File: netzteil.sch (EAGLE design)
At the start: 49 parts, among them X1 NEB21R

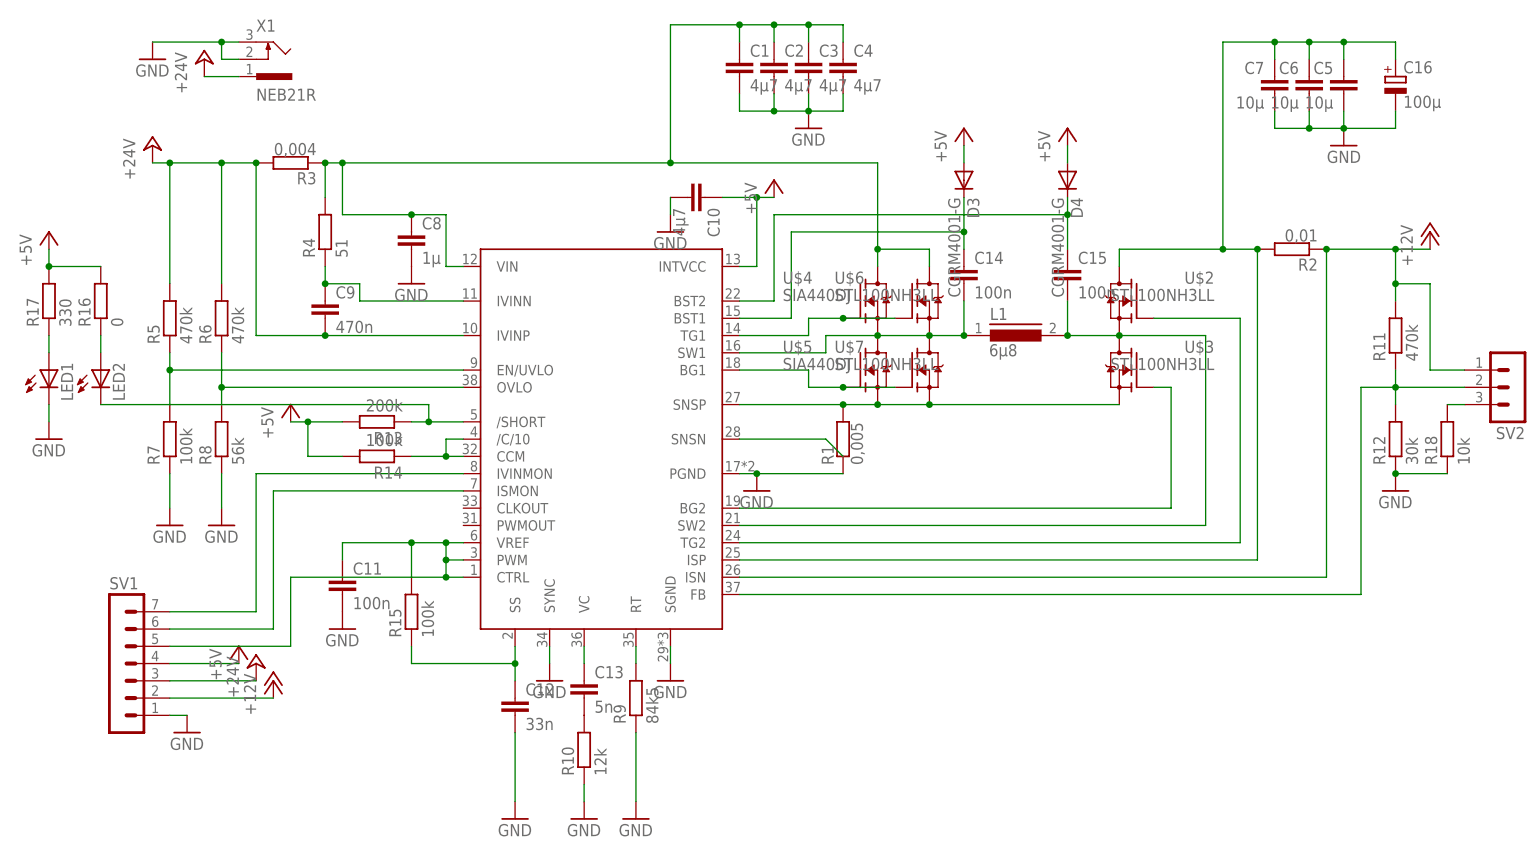
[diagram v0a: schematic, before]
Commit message: version 2
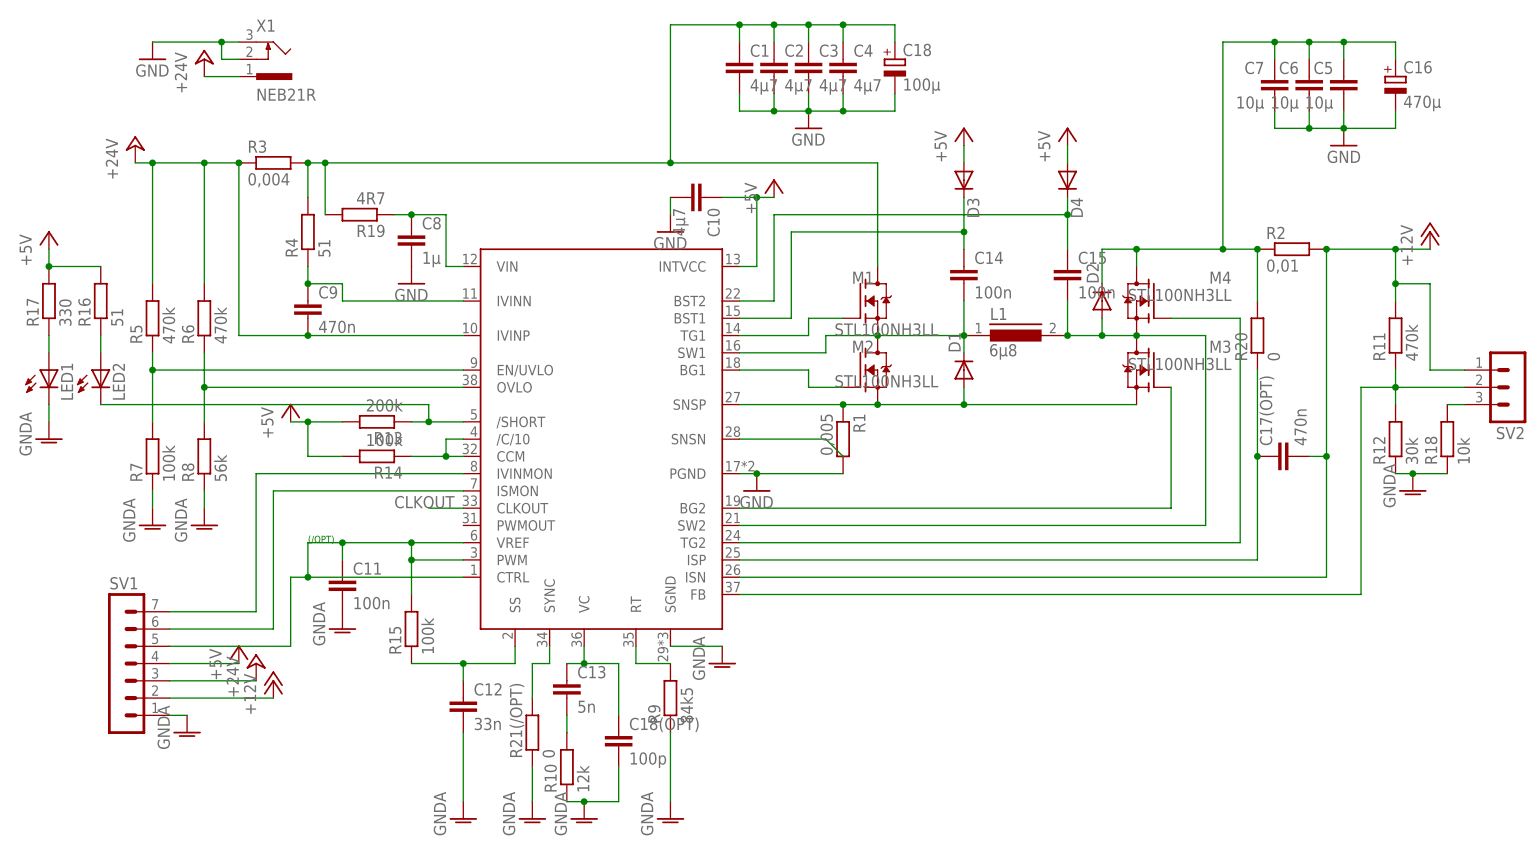
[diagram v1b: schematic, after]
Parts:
- removed U$2, U$3, U$6, U$7: STL100NH3LL, teile:STL100NH3LL
- removed U$4, U$5: SIA440DJ, teile:SIA440DJ
- added C17(OPT): 470n, resistor:C-EUC0805K
- added C18: 100µ, resistor:CPOL-EU153CLV-0605
- added C18(OPT): 100p, resistor:C-EUC0805K
- added D1, D2: (no value), diode:DIODE-SOD323-R
- added M1, M2, M3, M4: STL100NH3LL, teile:STL100NH3LL
- added R19: 4R7, resistor:R-EU_M0805
- added R20, R21(/OPT): 0, resistor:R-EU_M0805
- C16: value 100µ -> 470µ; device resistor:CPOL-EU153CLV-0807 -> resistor:CPOL-EU153CLV-1010
- D3, D4: value CGRM4001-G -> (none); device diode:CGRM4001-G -> diode:DIODE-SOD323-R
- R1, R2, R3: device resistor-shunt:BVS -> resistor:R-EU_R2512
- R16: value 0 -> 51
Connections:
- new net CLKOUT: U$1.CLKOUT
- new net GNDA: C11.2, C12.2, C18(OPT).2, LED1.C, R10.1, R12.1, R18.1, R21(/OPT).1, R7.1, R8.1, R9.1, SV1.1, U$1.SGND
- new net N$10: C17(OPT).1, R20.1, U$1.ISP
- new net N$9: C8.1, R19.1, U$1.VIN
- new net SYNC: R21(/OPT).2, U$1.SYNC
- net +12V: now also C17(OPT).2
- net BG1: now also M2.G; no longer U$5.G, U$7.G
- net BG2: now also M3.G; no longer U$3.G
- net GND: now also C18.-; no longer C11.2, C12.2, LED1.C, R10.1, R12.1, R18.1, R7.1, R8.1, R9.1, SV1.1, U$1.SGND, U$1.SYNC
- net ISP: now also D2.C, M4.D, R20.2; no longer U$1.ISP, U$2.D
- net N$8: now also C18(OPT).1
- net SNSP: now also D1.A, M2.S, M3.S; no longer U$3.S, U$5.S, U$7.S
- net SW1: now also D1.C, M1.S, M2.D; no longer U$4.S, U$5.D, U$6.S, U$7.D
- net SW2: now also D2.A, M3.D, M4.S; no longer U$2.S, U$3.D
- net TG1: now also M1.G; no longer U$4.G, U$6.G
- net TG2: now also M4.G; no longer U$2.G
- net VINN: now also C18.+, M1.D, R19.2; no longer C8.1, U$1.VIN, U$4.D, U$6.D
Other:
- note added: "(/OPT)"
- moved on the sheet: C12, C13, C9, R1, R10, R15, R2, R3, R4, R5, R6, R7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
